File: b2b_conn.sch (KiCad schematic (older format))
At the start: 3 parts

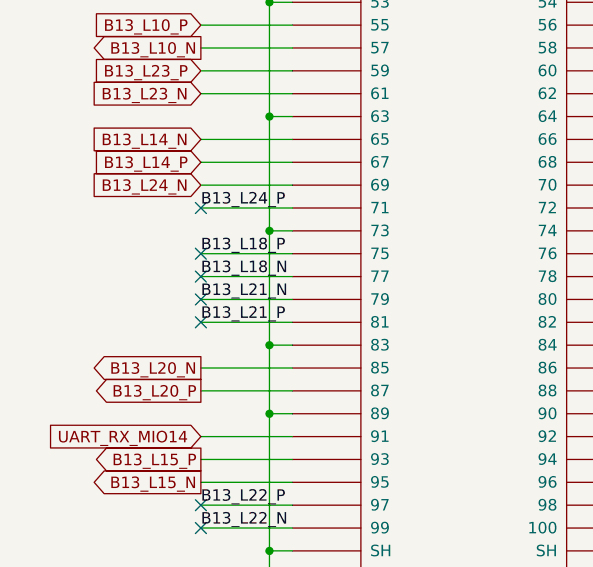
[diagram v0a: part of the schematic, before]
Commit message: cont. work; all connections done now
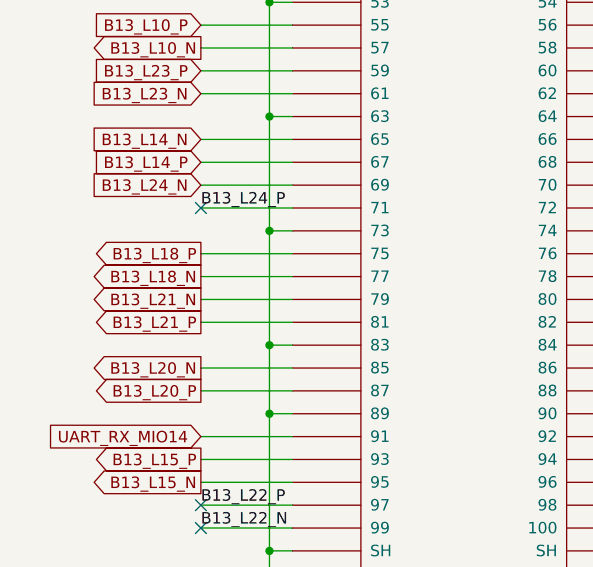
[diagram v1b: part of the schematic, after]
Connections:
- no-connect marks 18 -> 14
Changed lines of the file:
@@
 Wire Wire Line
 	1700 4700 1300 4700
-Text Label 1300 4900 0    50   ~ 0
-B13_L18_P
-Text Label 1300 5000 0    50   ~ 0
-B13_L18_N
 Wire Wire Line
 	1700 4900 1300 4900
 Wire Wire Line
 	1700 5000 1300 5000
-Text Label 1300 5100 0    50   ~ 0
-B13_L21_N
-Text Label 1300 5200 0    50   ~ 0
-B13_L21_P
 Wire Wire Line
 	1700 5100 1300 5100
@@
 B13_L24_N
 NoConn ~ 1300 4700
-NoConn ~ 1300 4900
-NoConn ~ 1300 5000
-NoConn ~ 1300 5100
-NoConn ~ 1300 5200
 $Comp
 L te0715:LSHM-130-04_JB3 JB3
@@
 Wire Wire Line
 	6800 3100 6550 3100
+Text GLabel 1300 5200 0    50   Output ~ 0
+B13_L21_P
+Text GLabel 1300 5100 0    50   Output ~ 0
+B13_L21_N
+Text GLabel 1300 5000 0    50   Output ~ 0
+B13_L18_N
+Text GLabel 1300 4900 0    50   Output ~ 0
+B13_L18_P
 $EndSCHEMATC
